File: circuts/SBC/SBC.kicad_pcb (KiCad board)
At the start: 2 copper layers, 108.2 x 121.5 mm, 372 parts, among them IC1 PIC16F15243-I_SS, J1 640456-3, J10 DE9_Plug, J11 buzzer, J13 Conn_01x04_Pin, J14 5v Power, J15 Barrel_Jack_MountingPin, J2 B5B-XH-A_LF__SN_, J3 Power, J4 DE9_Plug, J5 OSTTC060162, J6 XT60-M, J7 OSTTC060162, J8 DE9_Plug, J9 Conn_02x04_Odd_Even, Q1 MMBTA06, Q10 BC817, Q11 AO3400A, Q2 MMBTA06, Q3 MMBTA06, Q4 IRFS4227, Q5 MMBTA06, Q6 MMBTA06, Q7 MMBTA06, Q8 IRFS4227, SW1 SW_Push, SW2 SW_Push, SW3 SW_Push, SW4 SW_Push, SW5 SW_Push, SW6 rst, SW7 SW_Push, U1 UC3843, U10 ESP32-DEVKIT-V1, U12 L7805, U13 L7805, U14 L7809, U2 BTS7960B, U3 BTS7960B, U4 LM358DT, U5 AMS1117-3.3, U7 BTS7960B, U8 BTS7960B, U9 LM358DT

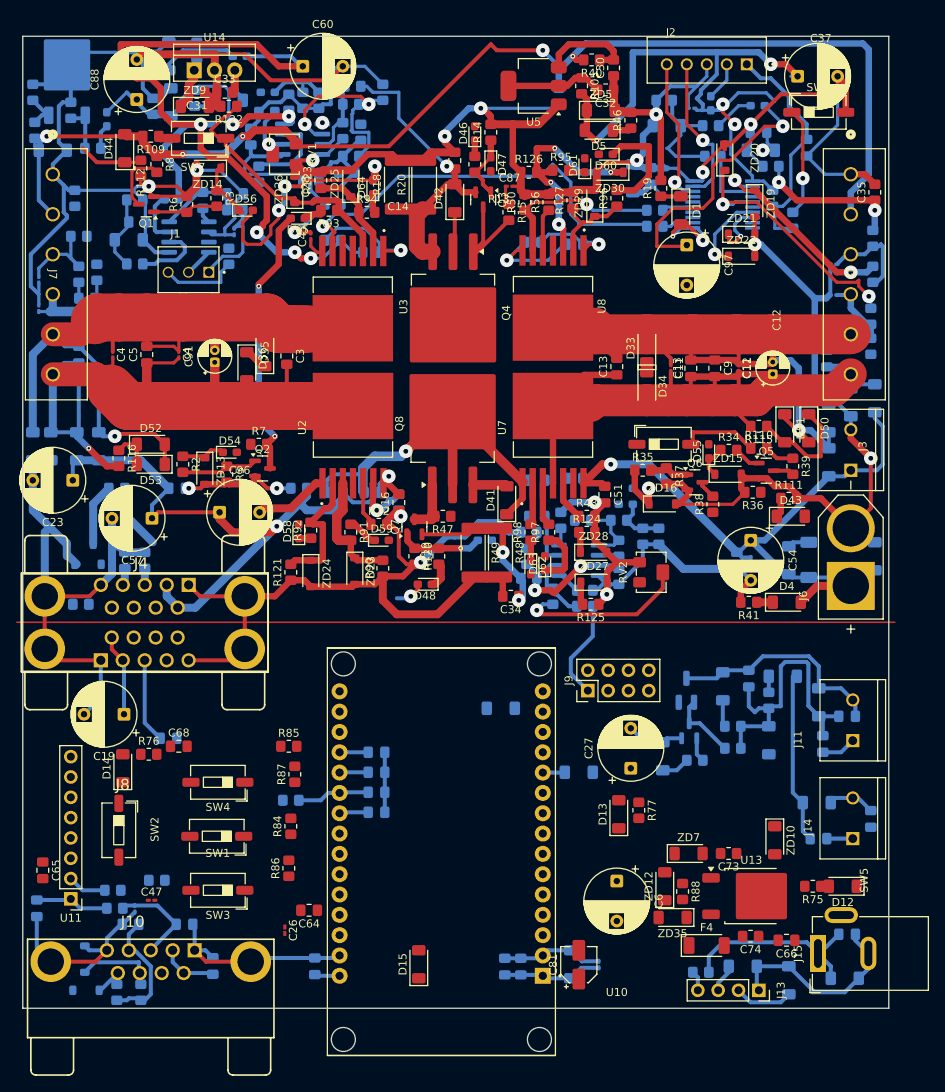
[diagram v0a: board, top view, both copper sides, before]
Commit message: siddyq has done almost done 7-25
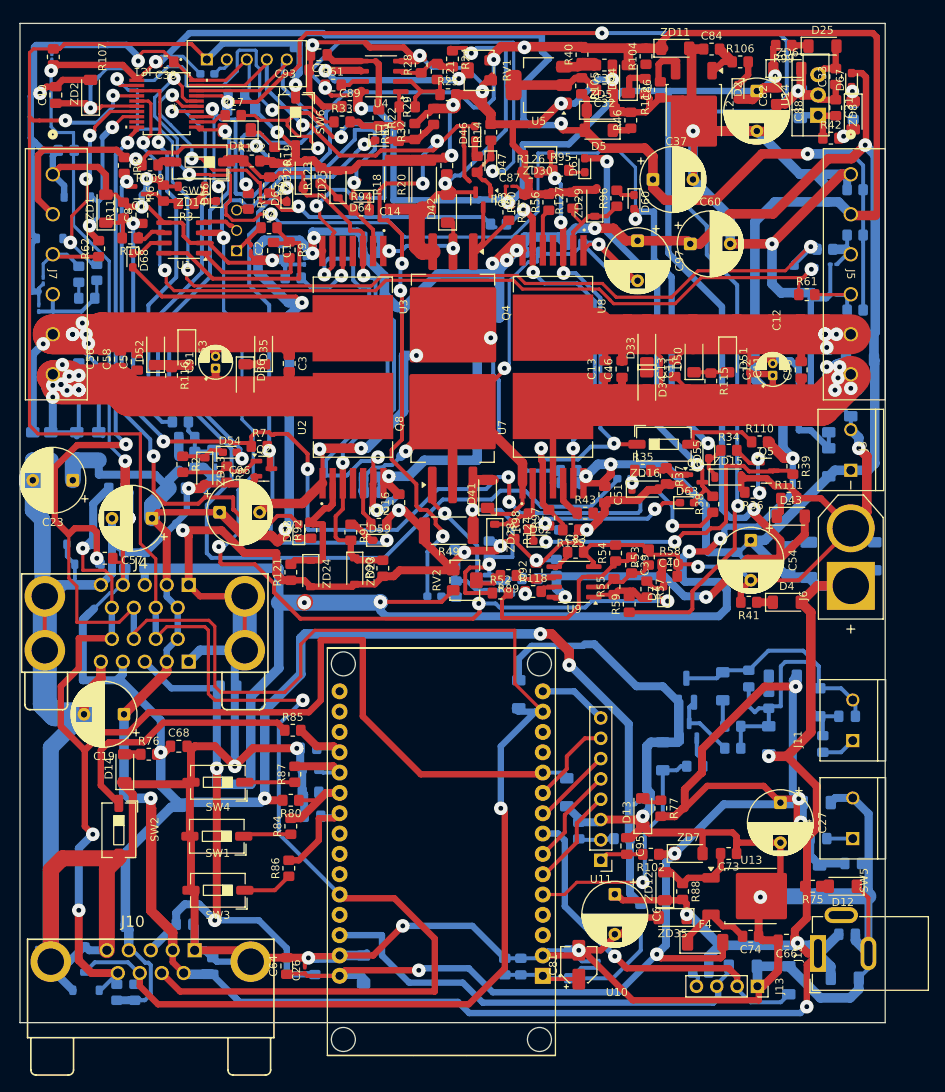
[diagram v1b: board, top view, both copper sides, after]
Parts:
- removed C4 (x2): 1nf, Capacitor_SMD:C_0201_0603Metric_Pad0.64x0.40mm_HandSolder
- removed the C9 at (249.0, 80.0)
- removed J9: Conn_02x04_Odd_Even, Connector_PinHeader_2.54mm:PinHeader_2x04_P2.54mm_Vertical
- removed R108: 1k, Resistor_SMD:R_0805_2012Metric_Pad1.20x1.40mm_HandSolder
- removed R48: 0.3, Resistor_SMD:R_2512_6332Metric_Pad1.40x3.35mm_HandSolder
- added C55: 2uf, Capacitor_SMD:C_0805_2012Metric_Pad1.18x1.45mm_HandSolder, F.Cu at (259.8, 80.2)
- added C56: 2uf, Capacitor_SMD:C_0805_2012Metric_Pad1.18x1.45mm_HandSolder, F.Cu at (172.6, 78.8)
- added C58: 2uf, Capacitor_SMD:C_0805_2012Metric_Pad1.18x1.45mm_HandSolder, F.Cu at (174.7, 78.9)
- C1, C10, C2, C21, C28, C38, C39, C40, C7, C8, C82, C83, C84, C86, C89, C92, C93, C95, D2, D25, D3, D67, D68, D7, IC1, R1, R10, R102, R104, R106, R107, R11, R118, R17, R22, R24, R25, R28, R29, R31, R32, R33, R4, R42, R51, R52, R53, R54, R55, R57, R58, R59, R61, R62, R65, R80, R89, R9, R99, U1, U12, U4, U9, ZD1, ZD11, ZD2, ZD6, ZD8: moved to F.Cu
- C34, C35, C45, C47, C65, D15, D48, J1, J8, Q7, R119, R120, R47, ZD10, ZD19, ZD20, ZD21, ZD22, ZD27, ZD9: moved to B.Cu
- C46: value 1nf -> 2uf; footprint Capacitor_SMD:C_0201_0603Metric_Pad0.64x0.40mm_HandSolder -> Capacitor_SMD:C_0805_2012Metric_Pad1.18x1.45mm_HandSolder; moved to F.Cu
- moved R107 91.6 mm to (166.3, 41.1), turned to -90 degrees
- moved C46 90.9 mm to (237.4, 80.1), turned to 90 degrees
- moved C10 88.0 mm to (166.6, 45.8), turned to 90 degrees
- moved R100 87.5 mm to (266.3, 47.9), turned to 90 degrees
- moved ZD22 86.5 mm to (165.9, 63.8), turned to 180 degrees
- moved ZD8 85.9 mm to (266.3, 48.4), turned to -90 degrees
- moved D66 85.0 mm to (182.0, 91.9), turned to -90 degrees
- moved ZD2 84.1 mm to (171.0, 45.7), turned to 90 degrees
- moved ZD21 83.2 mm to (169.3, 58.6), turned to 180 degrees
- moved R106 81.6 mm to (252.2, 41.7)
- moved C84 80.5 mm to (248.6, 40.1), turned to 0 degrees
- moved C36 80.2 mm to (166.1, 41.1), turned to 90 degrees
- moved R42 80.0 mm to (263.5, 51.2), turned to 0 degrees
- moved C31 79.9 mm to (264.1, 47.4), turned to -90 degrees
- moved D2 79.0 mm to (251.9, 45.5), turned to -90 degrees
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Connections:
- C46 pad 1: 5v+ -> M1_R
- C46 pad 2: GND -> M1_L
- SW6 pad 1: Net-(R108-Pad1) -> Mcler
- U10 pad 10: SDA2 -> int_a
- U10 pad 12: care -> care0
- U10 pad 13: care -> care0
- U10 pad 23: int_a -> unconnected-(U10-D25-Pad23)
- U10 pad 24: FSYC -> unconnected-(U10-D26-Pad24)
- U10 pad 27: care -> careuu
- U10 pad 3: care -> carett
- U10 pad 4: care -> carei
- U10 pad 6: unconnected-(U10-RX2-Pad6) -> SCL2
- U10 pad 7: unconnected-(U10-TX2-Pad7) -> SDA2
- U10 pad 9: SDL2 -> FSYC
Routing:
- net GND: track 856.4 -> 1379.4 mm, vias 21 -> 32
- net 5v+: track 211.0 -> 644.8 mm, vias 5 -> 17
- net 3.3v: track 125.3 -> 462.8 mm, vias 7 -> 11
- net HV: track 359.2 -> 687.4 mm, vias 9 -> 17
- net SCL: track 10.1 -> 266.8 mm, vias 0 -> 4
- net Mcler: track 32.4 -> 259.8 mm, vias 0 -> 4
- net M1_current_sen: track 8.56 -> 179.6 mm, vias 0 -> 3
- net 9v+: track 40.0 -> 203.6 mm, vias 2 -> 6
- net SDA: track 16.0 -> 169.3 mm, vias 0 -> 3
- net CS: track 0.00 -> 137.5 mm, vias 0 -> 5
- net M1_S1: track 0.00 -> 135.9 mm, vias 0 -> 5
- net Motor1_OFF: track 0.00 -> 128.2 mm, vias 0 -> 1
- net PWM: track 9.45 -> 129.9 mm, vias 0 -> 6
- net PGD: track 22.7 -> 123.4 mm, vias 3 -> 6
- net B1: track 24.8 -> 122.5 mm, vias 2 -> 3
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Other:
- board size 108.2 x 121.5 mm -> 108.2 x 124.9 mm
